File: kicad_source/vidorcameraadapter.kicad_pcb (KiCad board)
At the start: 2 copper layers, 62 x 47 mm, 53 parts, among them CN1 CONN_02X26, CN2 CONN_02X10, CN3 CONN_01X03

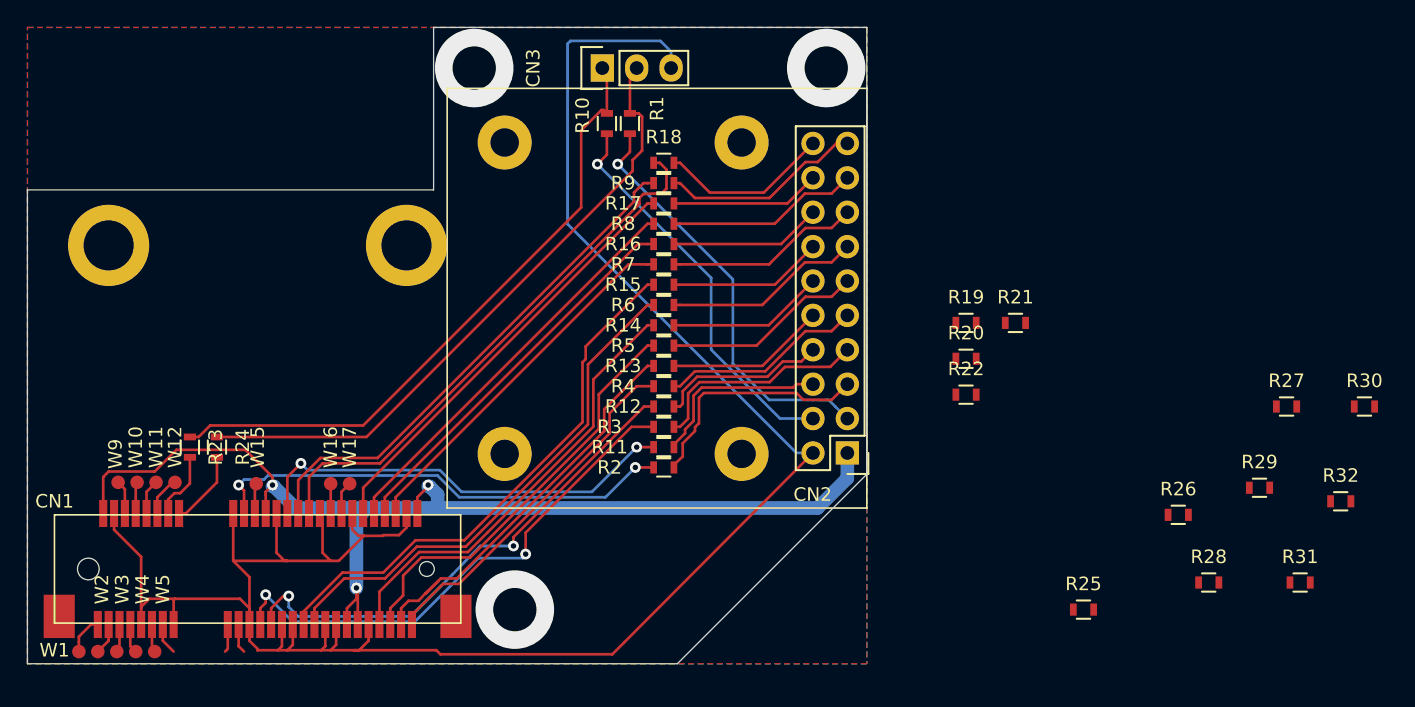
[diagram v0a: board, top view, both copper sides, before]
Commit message: placed all new parts in layout
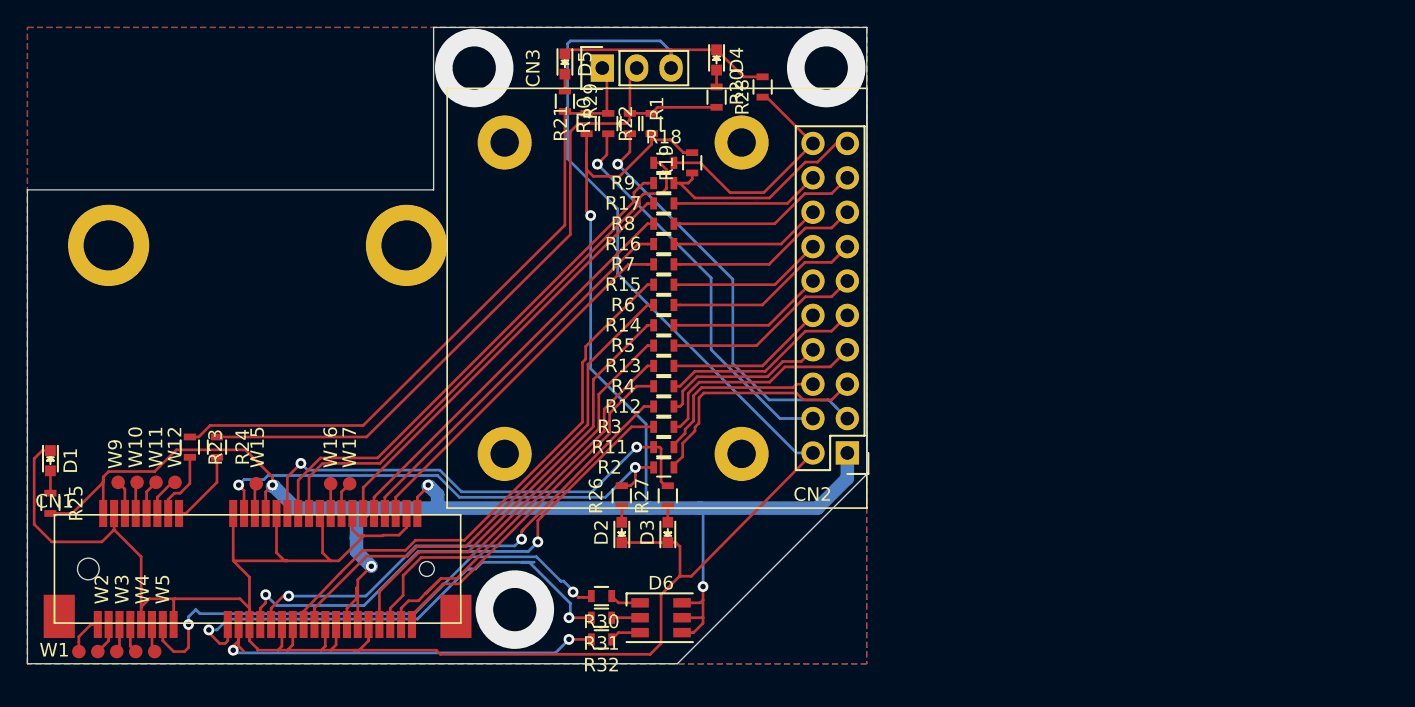
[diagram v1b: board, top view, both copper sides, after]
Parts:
- added D1: Led_Small, LEDs:LED_0603, F.Cu at (79.7, 122.0)
- added D2: Led_Small, LEDs:LED_0603, F.Cu at (121.9, 127.3)
- added D3: Led_Small, LEDs:LED_0603, F.Cu at (125.3, 127.3)
- added D4: Led_Small, LEDs:LED_0603, F.Cu at (128.9, 92.4)
- added D5: Led_Small, LEDs:LED_0603, F.Cu at (117.7, 92.7)
- added D6: LED_RGB, LEDs:LED_RGB_PLLC-6, F.Cu at (124.8, 133.6)
- moved R25 76.7 mm to (79.7, 125.2), turned to 270 degrees
- moved R29 58.7 mm to (117.7, 95.5), turned to 270 degrees
- moved R30 58.1 mm to (120.4, 132.0), turned to 180 degrees
- moved R32 55.5 mm to (120.4, 135.2), turned to 180 degrees
- moved R31 51.7 mm to (120.4, 133.6), turned to 180 degrees
- moved R28 51.1 mm to (128.9, 95.2), turned to 270 degrees
- moved R27 46.2 mm to (125.3, 124.6), turned to 90 degrees
- moved R26 41.1 mm to (121.9, 124.6), turned to 90 degrees
- moved R21 34.9 mm to (119.3, 97.1), turned to 90 degrees
- moved R22 30.7 mm to (124.1, 97.1), turned to 90 degrees
- moved R20 25.1 mm to (132.3, 94.4), turned to 90 degrees
- moved R19 23.4 mm to (127.1, 100.0), turned to 90 degrees
- moved R10 0.10 mm to (120.9, 97.1)
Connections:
- R25 pad 1: (no net) -> Net-(D1-Pad2)
- R26 pad 1: (no net) -> Net-(D2-Pad2)
- R27 pad 1: (no net) -> Net-(D3-Pad2)
- R28 pad 1: (no net) -> Net-(D4-Pad2)
- R29 pad 1: (no net) -> Net-(D5-Pad2)
- R30 pad 1: (no net) -> Net-(D6-Pad1)
- R31 pad 1: (no net) -> Net-(D6-Pad2)
- R32 pad 1: (no net) -> Net-(D6-Pad3)
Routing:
- net +3V3: track 82.0 -> 142.5 mm, vias 3 -> 5
- net GND: track 162.2 -> 201.0 mm
- net /LED_R: track 2.33 -> 39.0 mm, vias 0 -> 2
- net /LED_G: track 2.08 -> 37.2 mm, vias 0 -> 2
- net /LED_B: track 2.17 -> 31.2 mm, vias 0 -> 2
- net /SCL: track 47.0 -> 54.5 mm
- net /PWDN_R: track 12.7 -> 17.8 mm
- net /HREF: track 32.4 -> 36.1 mm
- net Net-(D6-Pad3): track 0.00 -> 2.31 mm
- net Net-(D6-Pad1): track 0.00 -> 2.31 mm
- net /VSYNC: track 34.8 -> 36.9 mm
- net Net-(D6-Pad2): track 0.00 -> 2.10 mm
- net /XCLK: track 37.7 -> 36.0 mm
- net Net-(D1-Pad2): track 0.00 -> 1.65 mm
- net /SDA: track 47.7 -> 49.3 mm
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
